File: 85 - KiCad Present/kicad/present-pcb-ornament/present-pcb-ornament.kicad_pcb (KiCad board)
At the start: 2 copper layers, 91.4 x 96.4 mm, 2 parts

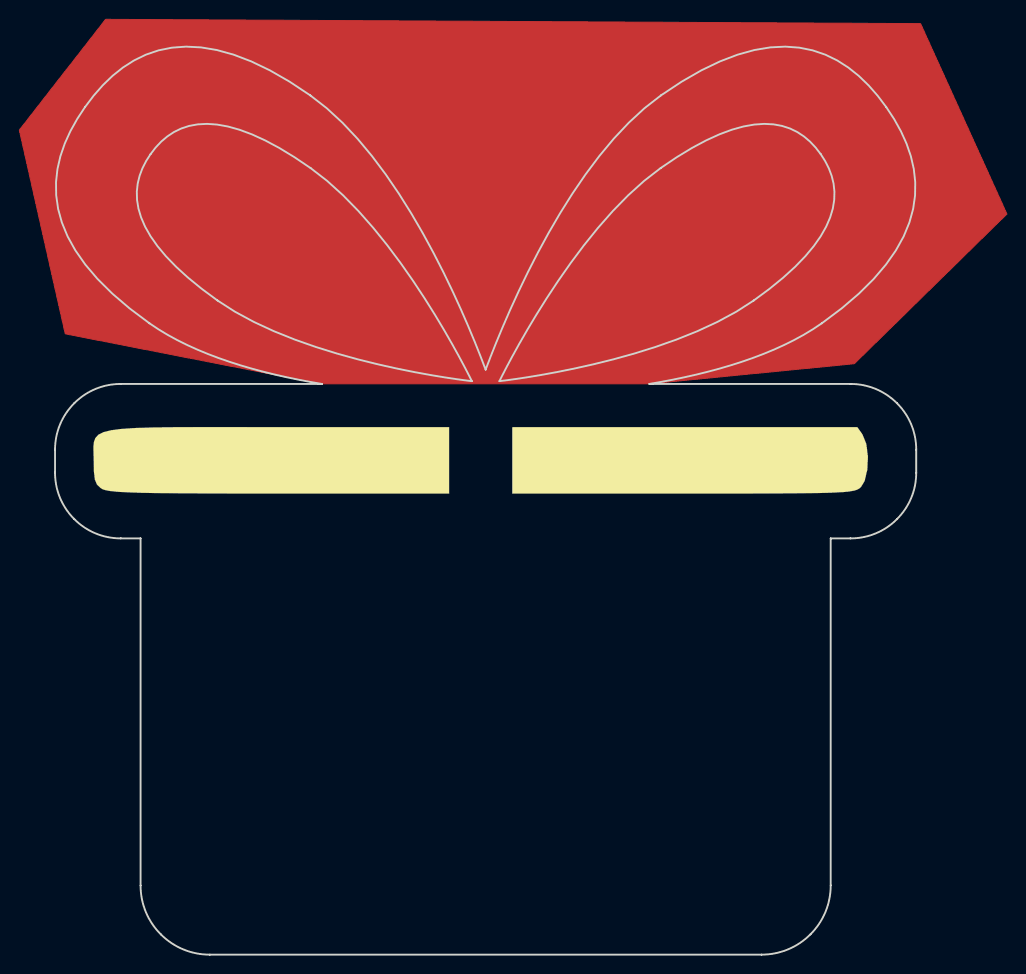
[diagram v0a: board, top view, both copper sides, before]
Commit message: post stream
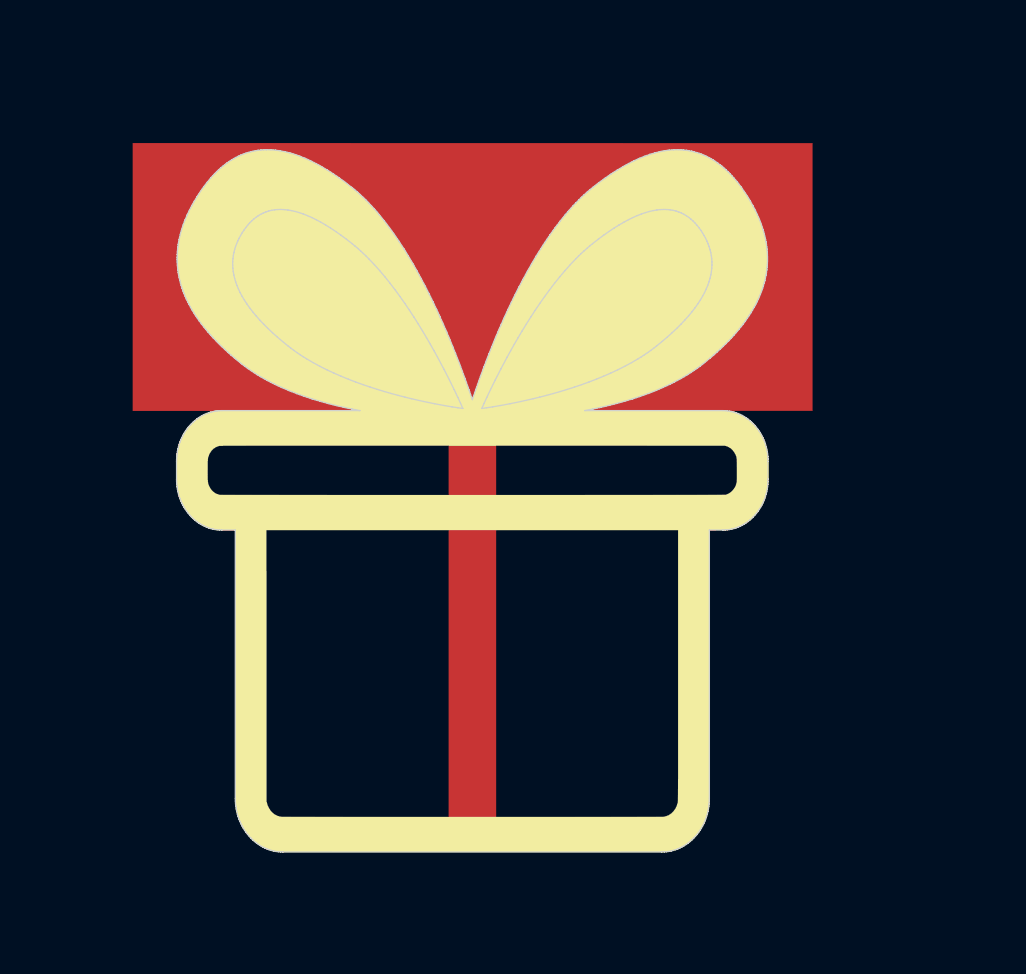
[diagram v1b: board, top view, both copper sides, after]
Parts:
- removed G*** (x2): LOGO, vector-files:inside zones
- added Ref**: Val**, svg2shen export:inky escaped, F.Cu at (157.7, 100.6)
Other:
- board size 91.4 x 96.4 mm -> 62.8 x 74.6 mm
